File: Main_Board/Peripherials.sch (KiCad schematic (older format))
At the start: 17 parts, among them J3 Conn_01x08, U5 MPU-6050

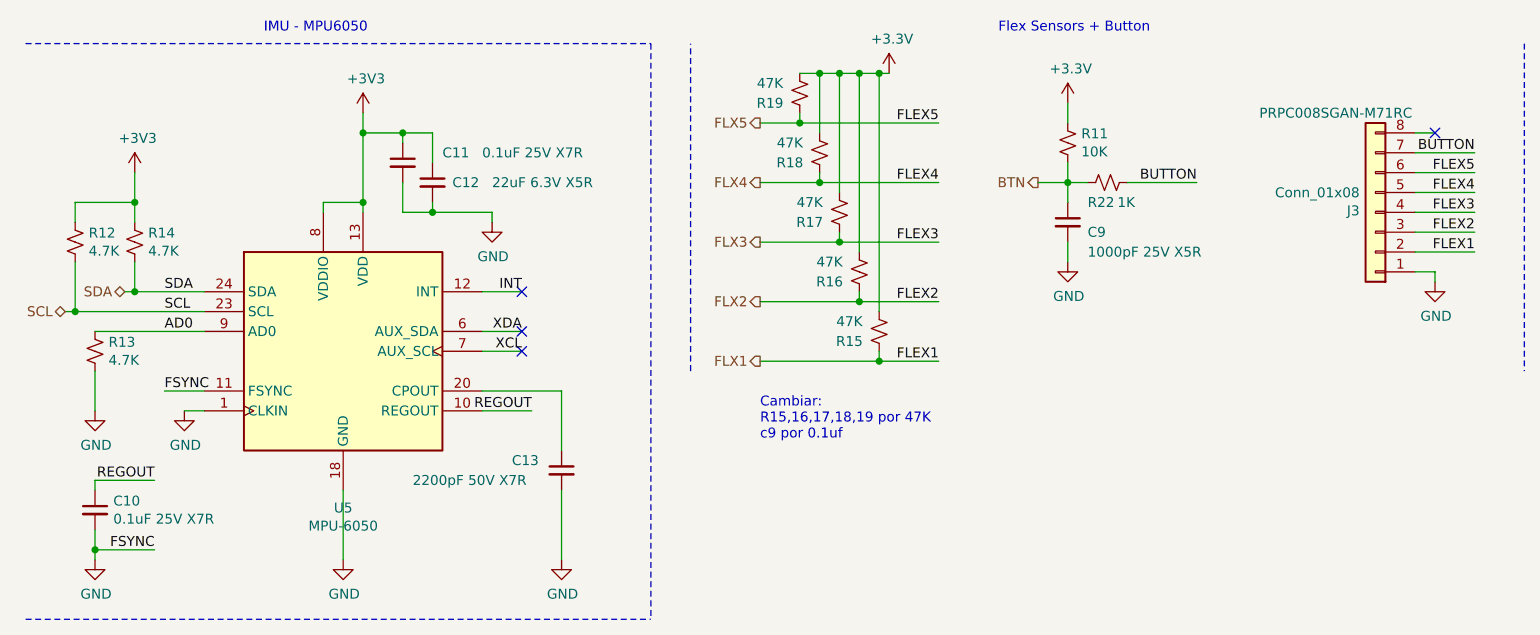
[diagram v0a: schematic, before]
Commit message: Rev 2.0 commit. INTI revision.
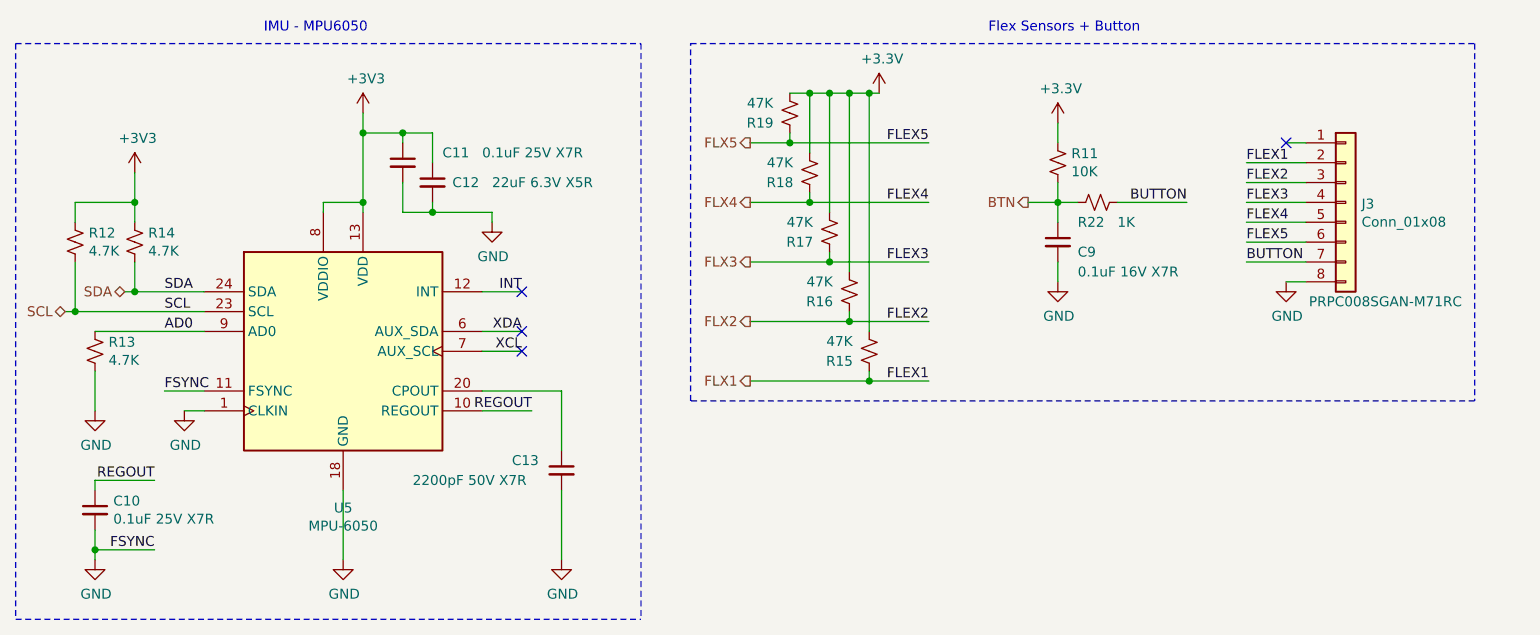
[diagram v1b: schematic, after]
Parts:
- C9: value 1000pF 25V X5R -> 0.1uF 16V X7R; *Digikey 06033C102KAT2A -> 0603YC104K4T2A
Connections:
- net GND: now also J3.8 (Pin_8); no longer J3.1 (Pin_1)
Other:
- note removed: "Cambiar:\nR15,16,17,18,19 por 47K\nc9 por 0.1uf"
- moved on the sheet: C9, J3, R11, R15, R16, R17, R18, R19, R22
